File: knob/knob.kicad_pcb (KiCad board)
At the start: 2 copper layers, 94.1 x 82.7 mm, 10 parts, among them SW1 SW_Push, SW2 SW_Push, SW3 SW_Push, SW4 SW_Push, SW5 SW_Push, SW6 SW_Push, SW7 RotaryEncoder_Switch, SW8 RotaryEncoder_Switch

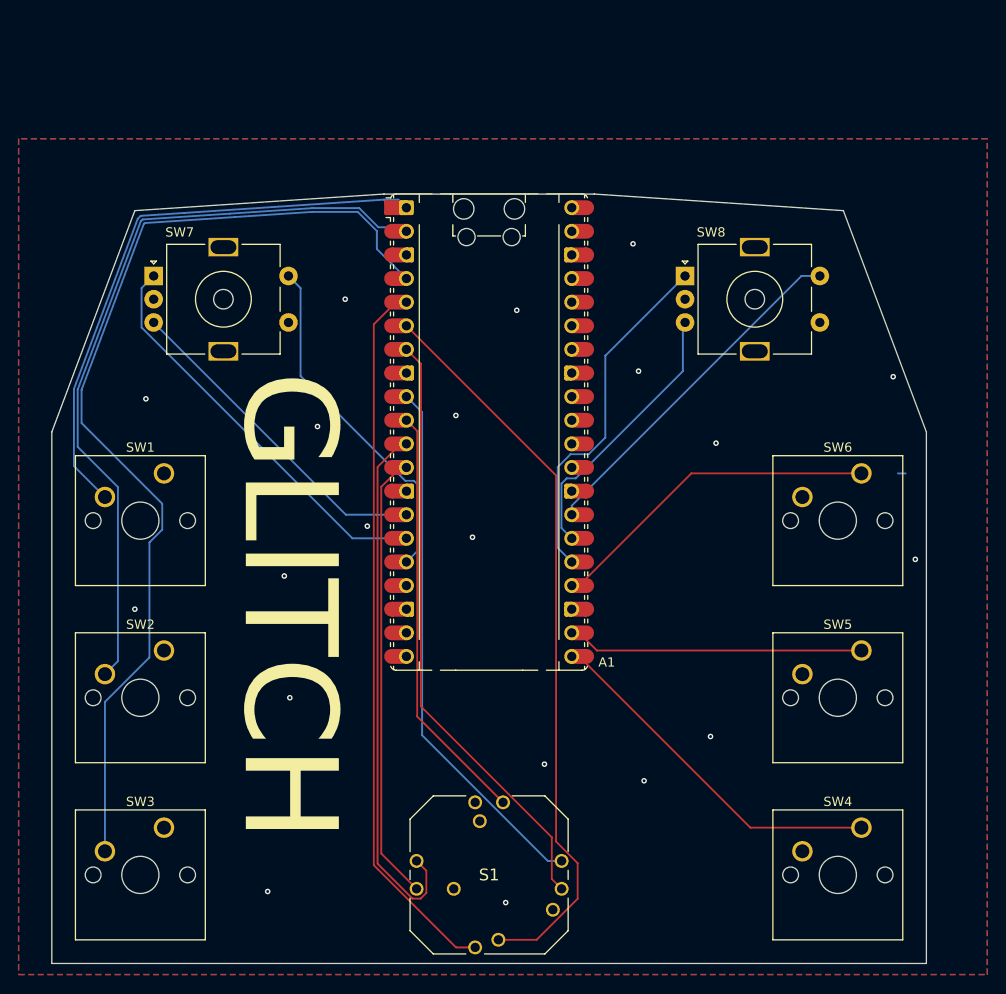
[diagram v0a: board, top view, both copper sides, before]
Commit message: sync
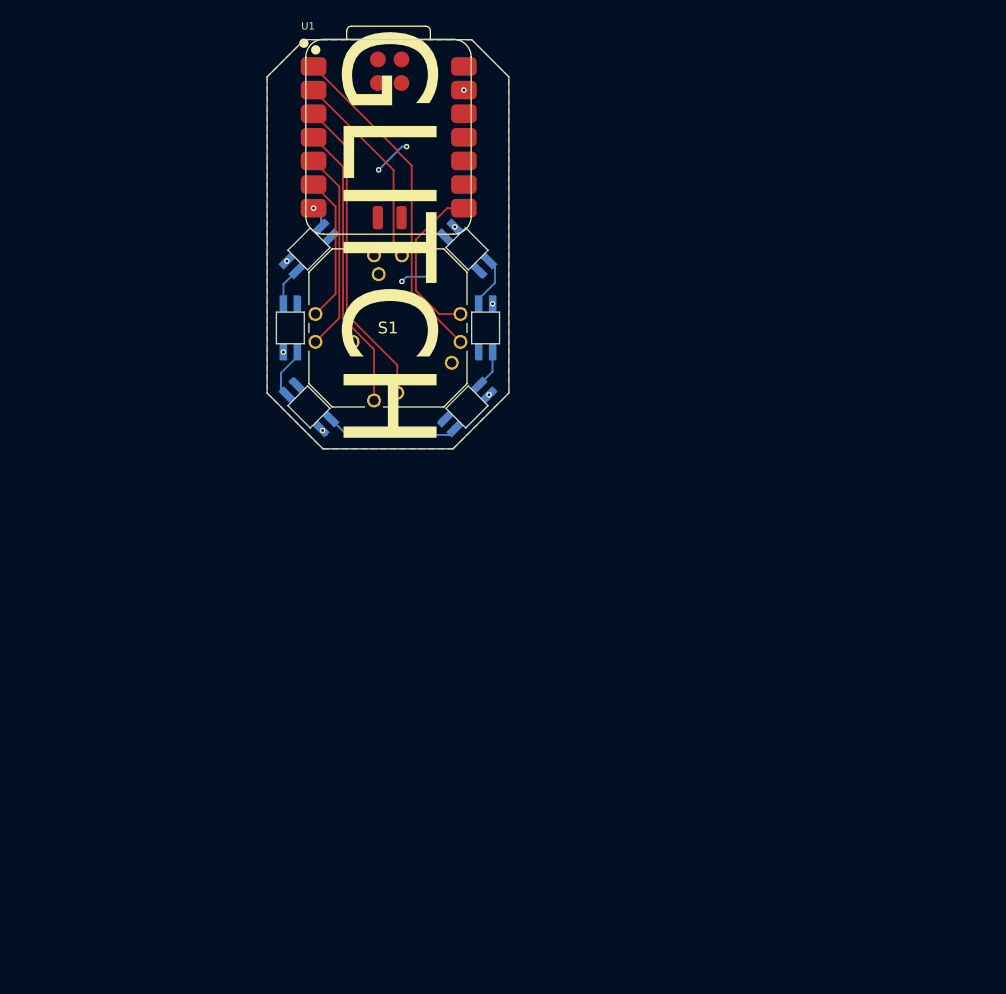
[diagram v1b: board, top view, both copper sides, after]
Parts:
- removed A1: RaspberryPi_Pico, Module:RaspberryPi_Pico_Common_Unspecified
- removed SW1, SW2, SW3, SW4, SW5, SW6: SW_Push, Button_Switch_Keyboard:SW_Cherry_MX_1.00u_PCB
- removed SW7, SW8: RotaryEncoder_Switch, Rotary_Encoder:RotaryEncoder_Alps_EC11E-Switch_Vertical_H20mm_MountingHoles
- added D1: SK6812MINI, cheyao macropad main PCB-third_party_neopixel.petty:SK6812MINI-E, B.Cu at (123.5, 56.5)
- added D2: SK6812MINI, cheyao macropad main PCB-third_party_neopixel.petty:SK6812MINI-E, B.Cu at (121.5, 65.0)
- added D3: SK6812MINI, cheyao macropad main PCB-third_party_neopixel.petty:SK6812MINI-E, B.Cu at (123.5, 73.5)
- added D4: SK6812MINI, cheyao macropad main PCB-third_party_neopixel.petty:SK6812MINI-E, B.Cu at (140.5, 73.5)
- added D5: SK6812MINI, cheyao macropad main PCB-third_party_neopixel.petty:SK6812MINI-E, B.Cu at (142.5, 65.0)
- added D6: SK6812MINI, cheyao macropad main PCB-third_party_neopixel.petty:SK6812MINI-E, B.Cu at (140.5, 56.5)
- added U1: XIAO-RP2040-SMD, Seeed Studio XIAO Series Library:XIAO-RP2040-SMD, F.Cu at (132.0, 44.5)
- moved S1 59.8 mm to (132.0, 65.0)
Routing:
- net Net-(A1-GPIO2): track 107.3 -> 0.00 mm
- net Net-(A1-GPIO1): track 82.0 -> 0.00 mm
- net Net-(A1-GPIO0): track 62.0 -> 0.00 mm
- net A: track 77.2 -> 31.0 mm
- net PUSH: track 79.6 -> 33.7 mm
- net Net-(A1-GPIO11): track 44.0 -> 0.00 mm
- net D: track 57.7 -> 15.8 mm
- net ENC0B: track 57.7 -> 17.9 mm
- net Net-(A1-GPIO19): track 38.2 -> 0.00 mm
- net Net-(A1-GPIO16): track 38.0 -> 0.00 mm
- net Net-(A1-GPIO21): track 37.9 -> 0.00 mm
- net Net-(A1-GPIO12): track 37.5 -> 0.00 mm
- net Net-(A1-GPIO18): track 36.2 -> 0.00 mm
- net Net-(A1-GPIO10): track 35.7 -> 0.00 mm
- net Net-(A1-GPIO17): track 31.1 -> 0.00 mm
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- added copper zone on F.Cu, net +5V
- removed copper zone on F.Cu, net GND
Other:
- board size 94.1 x 82.7 mm -> 26 x 44 mm
